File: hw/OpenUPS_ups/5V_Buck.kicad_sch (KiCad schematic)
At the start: 24 parts, among them U201 TPS51397A, U202 INA180A3

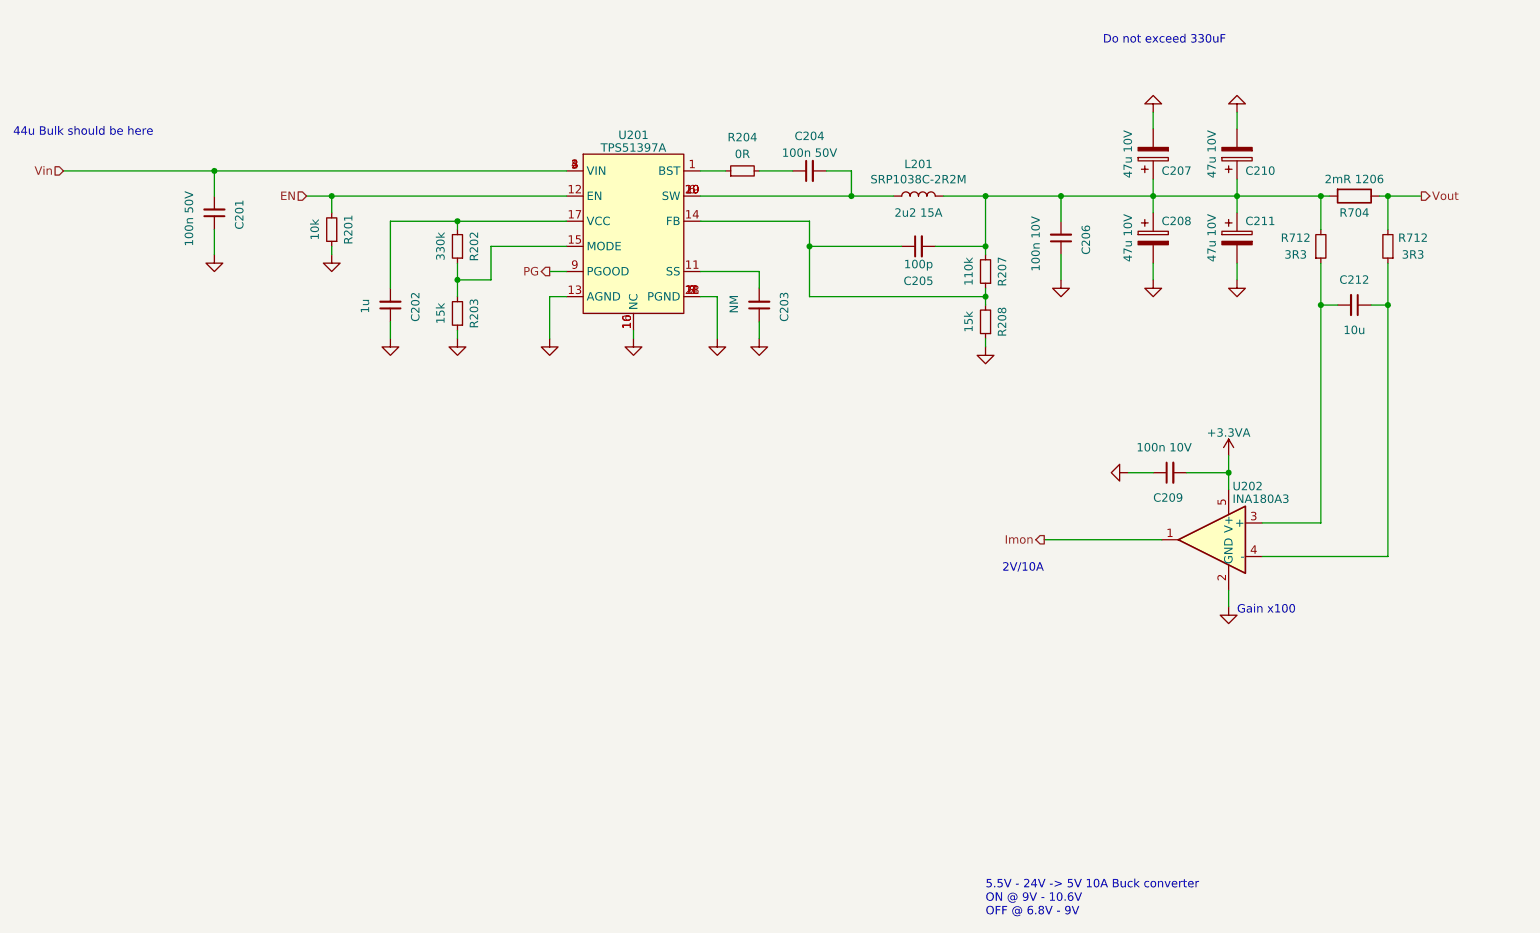
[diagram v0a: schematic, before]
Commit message: PCB placement
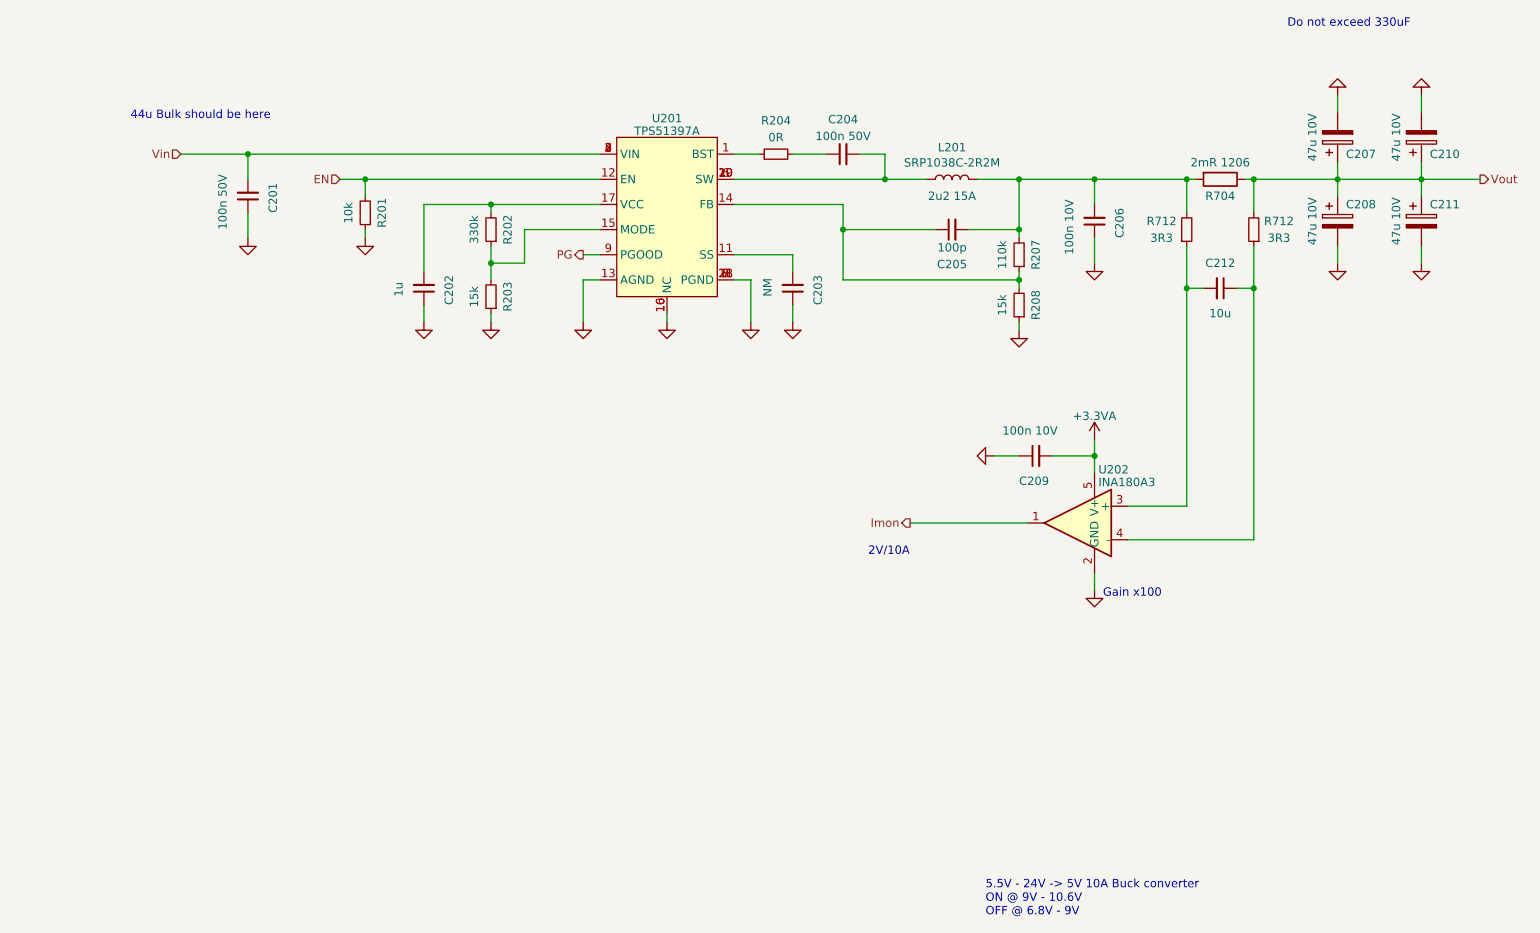
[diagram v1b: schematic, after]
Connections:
- net Vout: now also C207.1, C208.1, C210.1, C211.1
- net at C205.2, C206.2, L201.2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: no longer C207.1, C208.1, C210.1, C211.1
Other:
- moved on the sheet: C201, C202, C203, C204, C205, C206, C207, C208, C209, C210, C211, C212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
